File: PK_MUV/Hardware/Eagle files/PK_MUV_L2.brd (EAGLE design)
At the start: 28.1 x 21.3 mm, 5 parts

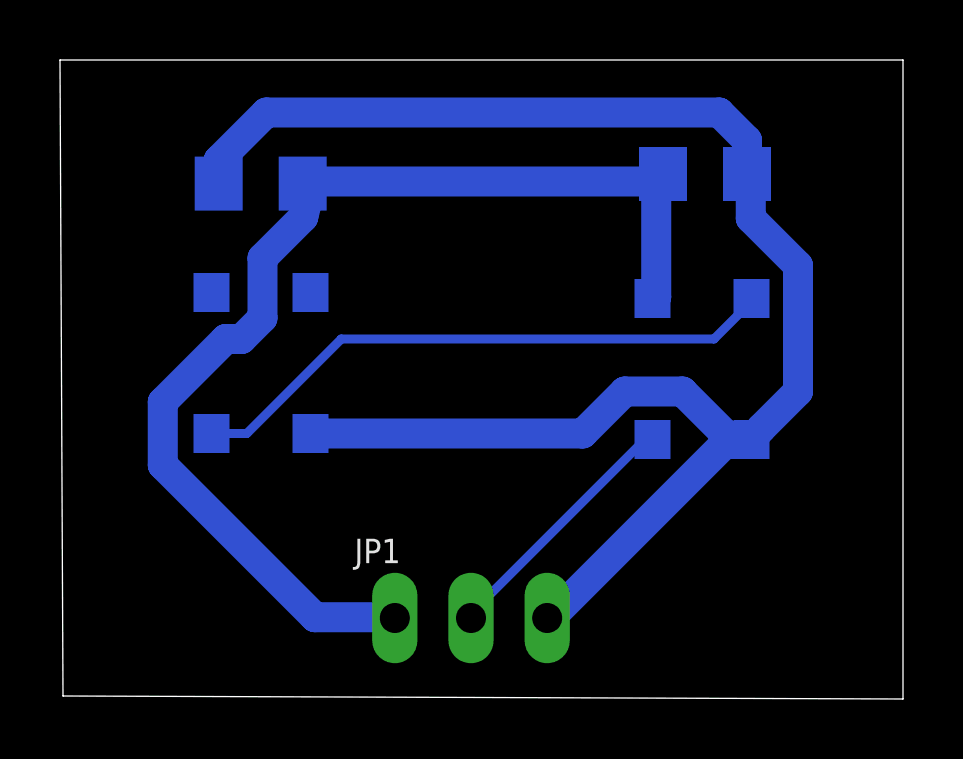
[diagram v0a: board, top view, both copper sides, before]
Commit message: update batt
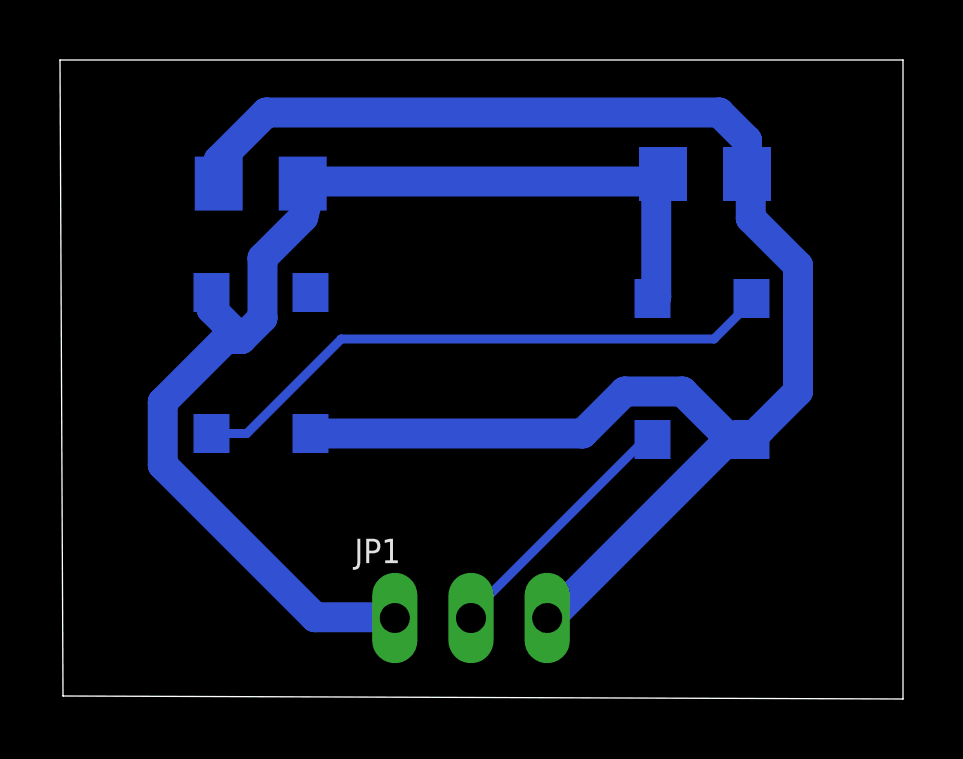
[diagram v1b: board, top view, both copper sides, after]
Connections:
- removed net VDD: LED2.1-VDD
- net BAT: now also LED2.1-VDD
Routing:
- net BAT: track 38.0 -> 39.9 mm
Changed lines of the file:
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@@
 <wire x1="8.156175" y1="16.546175" x2="7.99" y2="16.71235" width="1" layer="16"/>
 <wire x1="7.99" y1="16.71235" x2="7.99" y2="17.08" width="1" layer="16"/>
+<contactref element="LED2" pad="1-VDD"/>
+<wire x1="4.95" y1="13.45" x2="4.95" y2="12.9" width="1" layer="16"/>
+<wire x1="4.95" y1="12.9" x2="5.95" y2="11.9" width="1" layer="16"/>
 </signal>
 <signal name="GND" class="1">
@@
 <wire x1="13.475" y1="2.625" x2="13.6" y2="2.6" width="0.3" layer="16"/>
 </signal>
-<signal name="VDD">
-<contactref element="LED2" pad="1-VDD"/>
-</signal>
 <signal name="N$3">
